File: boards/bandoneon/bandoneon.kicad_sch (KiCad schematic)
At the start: 6 parts, among them J1 2D JOYSTICK

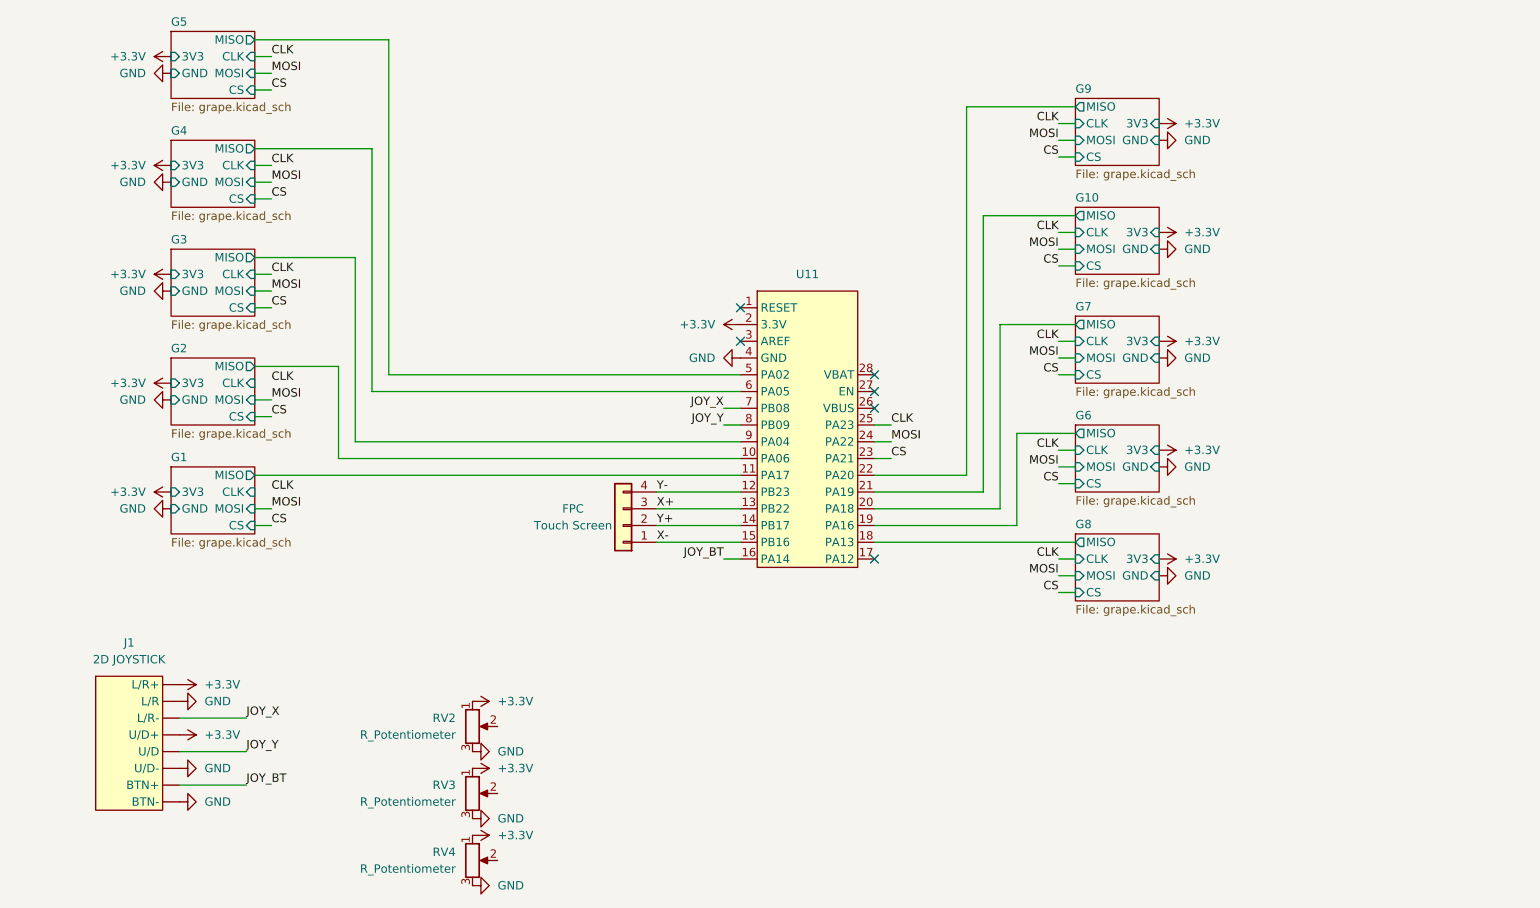
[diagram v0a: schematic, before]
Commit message: Schamtic complete
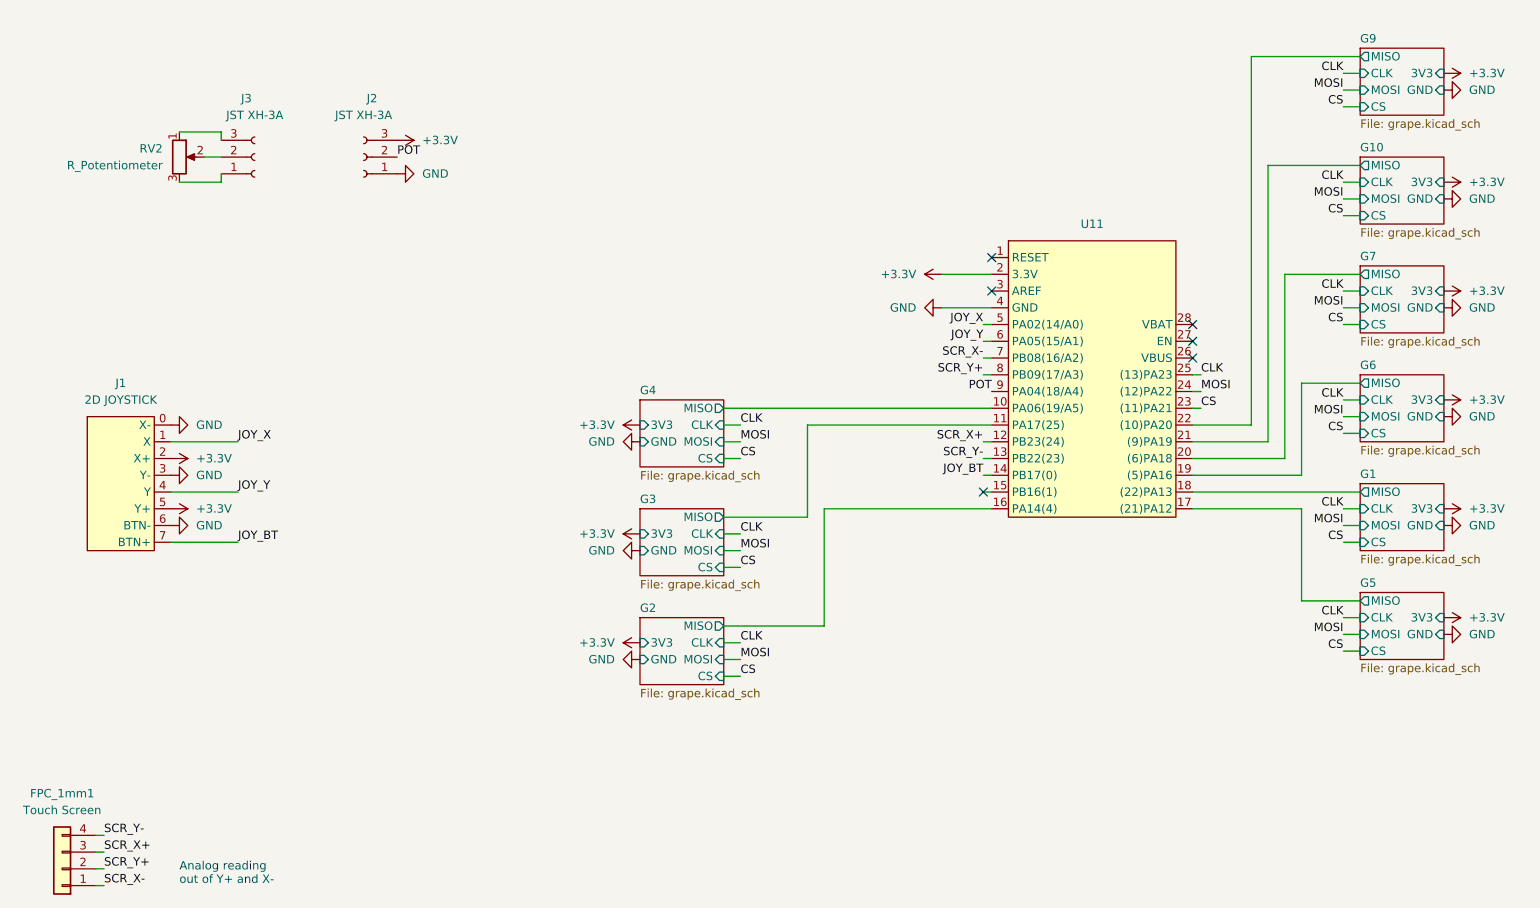
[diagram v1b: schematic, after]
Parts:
- removed RV3, RV4: R_Potentiometer, symbol Device:R_Potentiometer
- added J2: JST XH-3A, Connector_JST:JST_XH_B3B-XH-A_1x03_P2.50mm_Vertical, symbol Connector:Conn_01x03_Socket
- added J3: JST XH-3A, symbol Connector:Conn_01x03_Socket
- J1: footprint (none) -> Library:Adafruit (512) Analog 2-axis Thumb Joystick with Select Button
- renumbered FPC to FPC_1mm1
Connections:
- net G8/MISO is gone; now on net G1/MISO: U11.18 ((22)PA13)
- net +3.3V: now also J1.2 (X+), J1.5 (Y+), J2.3 (Pin_3); no longer J1. (U/D-), RV2.1
- net G1/MISO: no longer U11.11 (PA17)
- net G2/MISO: now also U11.16 (PA14(4)); no longer U11.10 (PA06)
- net G3/MISO: now also U11.11 (PA17(25)); no longer U11.9 (PA04)
- net G4/MISO: now also U11.10 (PA06(19/A5)); no longer U11.6 (PA05)
- net G5/MISO: now also U11.17 ((21)PA12); no longer U11.5 (PA02)
- net GND: now also J1.0 (X-), J1.3 (Y-), J1.6 (BTN-), J2.1 (Pin_1); no longer J1. (U/D-), RV2.3
- net JOY_BT: now also J1.7 (BTN+), U11.14 (PB17(0)); no longer J1. (U/D-), U11.16 (PA14)
- net JOY_X: now also J1.1 (X), U11.5 (PA02(14/A0)); no longer J1. (U/D-), U11.7 (PB08)
- net JOY_Y: now also J1.4 (Y), U11.6 (PA05(15/A1)); no longer J1. (U/D-), U11.8 (PB09)
- net at RV2.2: now also J3.2 (Pin_2)
- net X+ renamed SCR_X+
- net SCR_X+: now also U11.12 (PB23(24)); no longer U11.13 (PB22)
- net X-: no longer names the net of U11.15 (PB16(1))
- net X-: no longer FPC_1mm1.1 (Pin_1)
- net Y+ renamed SCR_Y+
- net SCR_Y+: now also U11.8 (PB09(17/A3)); no longer U11.14 (PB17)
- net Y- renamed SCR_Y-
- net SCR_Y-: now also U11.13 (PB22(23)); no longer U11.12 (PB23)
- new net: J3.3 (Pin_3), RV2.1
- new net: J3.1 (Pin_1), RV2.3
- new net POT: J2.2 (Pin_2), U11.9 (PA04(18/A4))
- new net SCR_X-: FPC_1mm1.1 (Pin_1), U11.7 (PB08(16/A2))
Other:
- removed sheet G8
- note added: "Analog reading out of Y+ and X-"
- moved on the sheet: FPC_1mm1, RV2, U11
